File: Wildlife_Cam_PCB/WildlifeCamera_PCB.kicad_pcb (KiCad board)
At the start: 2 copper layers, 45 parts, among them J1 PIR, J2 TRIG, J3 RTC_DS3231, J4 PROG, J5 PROG_EN, J6 LOGO1, J7 LOGO2, Q1 2N3904, Q2 2N3904, Q3 2N3904, SW1 ON/OFF, SW2 TRIGGER, U1 MCP1826S-3302, U2 BQ24210, U3 ESP32_CAM

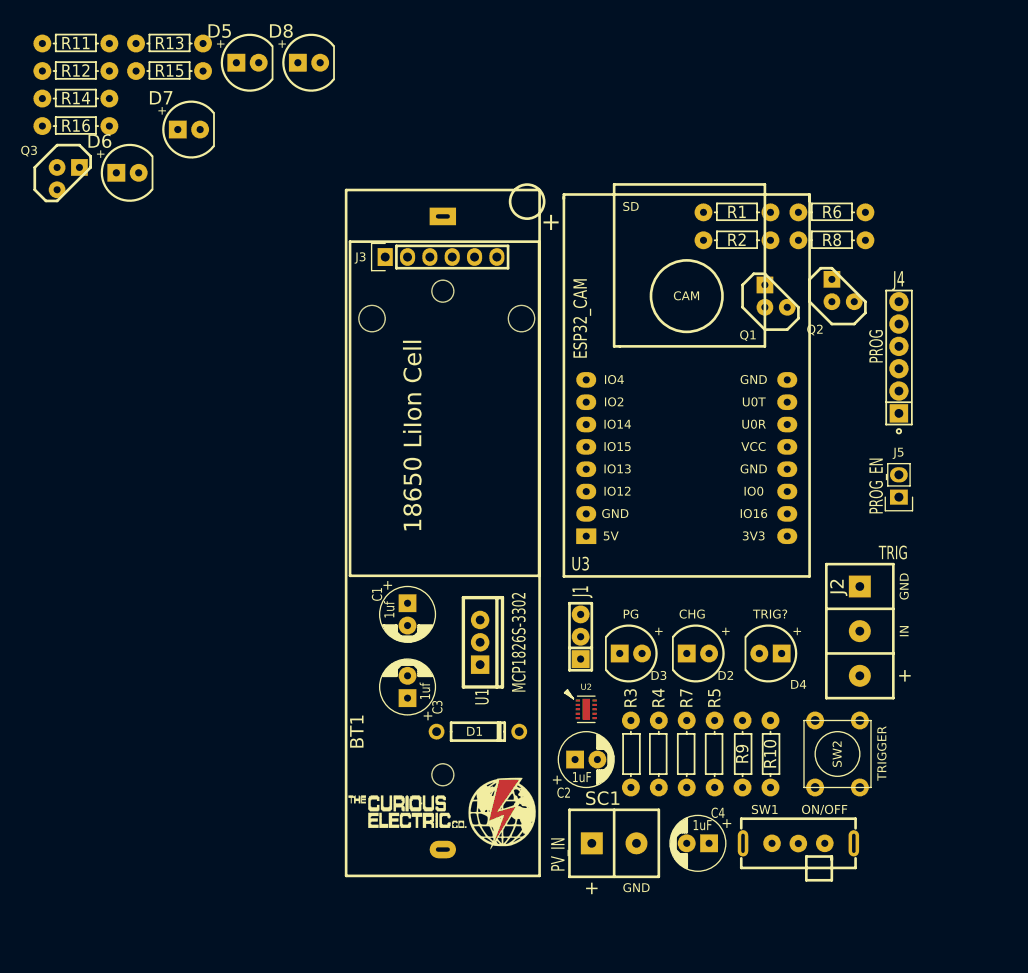
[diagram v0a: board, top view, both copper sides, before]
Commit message: Update of PCB
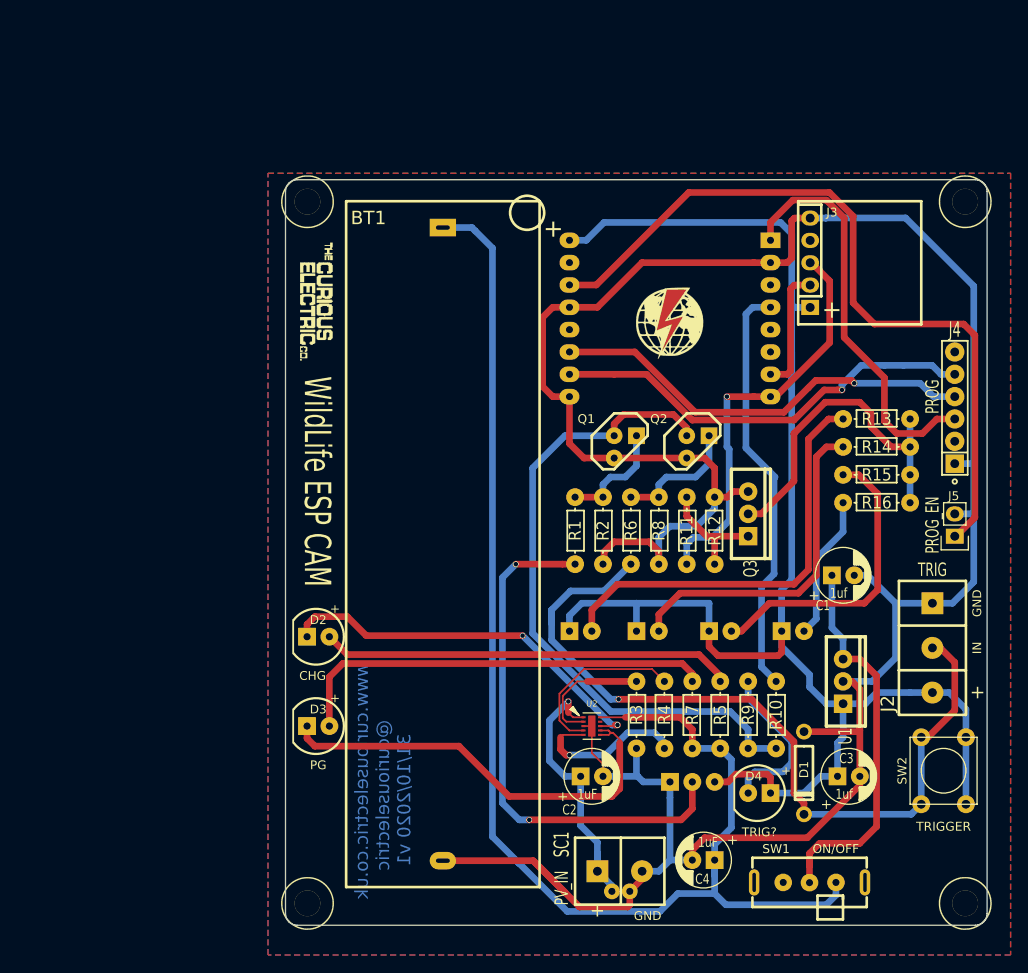
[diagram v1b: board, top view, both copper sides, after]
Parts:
- added J8: PCB, REInnovationFootprint:PCB_Wildlife_Cam, F.Cu at (198.8, 146.1)
- D5, D6, D7, D8, J1: moved to B.Cu
- J3: footprint REInnovationFootprint:TH_RTC_MODULE -> REInnovationFootprint:TH_RTC_MODULE_SM
- Q3: value 2N3904 -> BD135; footprint REInnovationFootprint:TO92-EBC_large_pad -> REInnovationFootprint:TO220_BD135
- SC1: footprint REInnovationFootprint:SIL-2_screw_terminal -> REInnovationFootprint:SIL_2_screw_+_JST_2mm
- moved R16 100.6 mm to (171.4, 90.2)
- moved R14 99.3 mm to (171.4, 83.8)
- moved R15 92.6 mm to (171.4, 87.0)
- moved R13 91.0 mm to (171.4, 80.6)
- moved R12 89.5 mm to (153.0, 93.3), turned to 90 degrees
- moved R11 88.9 mm to (149.9, 93.3), turned to 270 degrees
- moved Q3 86.2 mm to (156.8, 91.4)
- moved D8 84.9 mm to (161.9, 104.8)
- moved D7 83.1 mm to (153.7, 104.8)
- moved D6 78.8 mm to (145.4, 104.8)
- moved D5 74.9 mm to (137.8, 104.8)
- moved J6 62.9 mm to (109.9, 60.3), turned to 270 degrees
- moved J3 61.3 mm to (176.5, 55.9), turned to 180 degrees
- moved J7 58.9 mm to (148.6, 73.8)
- moved C3 51.2 mm to (168.3, 121.3), turned to 0 degrees
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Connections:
- D1 pad 2: +3V3 -> GND
- J3 pad 1: Net-(J3-Pad1) -> +3V3
- J3 pad 2: /ALARM -> /I2C_DAT
- J3 pad 4: /I2C_DAT -> Net-(J3-Pad4)
- J3 pad 5: +3V3 -> GND
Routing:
- net GND: track 0.00 -> 299.4 mm
- net +3V3: track 0.00 -> 182.7 mm
- net VCC: track 0.00 -> 155.9 mm
- net Net-(D1-Pad1): track 0.00 -> 92.4 mm, vias 0 -> 1
- net /PROG_EN: track 0.00 -> 86.8 mm
- net /TRIG: track 0.00 -> 75.5 mm
- net Net-(D3-Pad1): track 0.00 -> 62.9 mm
- net Net-(J1-Pad2): track 0.00 -> 60.5 mm, vias 0 -> 2
- net /U0T: track 0.00 -> 49.3 mm, vias 0 -> 1
- net /U0R: track 0.00 -> 48.9 mm, vias 0 -> 1
- net Net-(D3-Pad2): track 0.00 -> 48.9 mm
- net Net-(D5-Pad2): track 0.00 -> 48.7 mm
- net Net-(R10-Pad1): track 0.00 -> 48.0 mm
- net Net-(D2-Pad2): track 0.00 -> 46.9 mm
- net /I2C_CLK: track 0.00 -> 46.7 mm, vias 0 -> 1
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- added copper zone on B.Cu, net GND
- added copper zone on F.Cu, net GND
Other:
- board outline added: 79.8 x 84.8 mm
- board text added: "31/10/2020 v1"
- board text added: "@curiouselectric"
- board text added: "FLASH"
- board text added: "PIR"
- board text added: "WildLife ESP CAM"
- board text added: "www.curiouselectric.co.uk"
